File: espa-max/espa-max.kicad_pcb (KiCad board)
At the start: 2 copper layers, 44.1 x 47.5 mm, 39 parts, among them J1 Conn_01x11_Pin, J3 RJ45_LED_Shielded_x2, J5 AudioPlug2, U1 ESP32-S3-MINI-1-N8, U2 ESD7104MUTAG, U3 AP63203WU

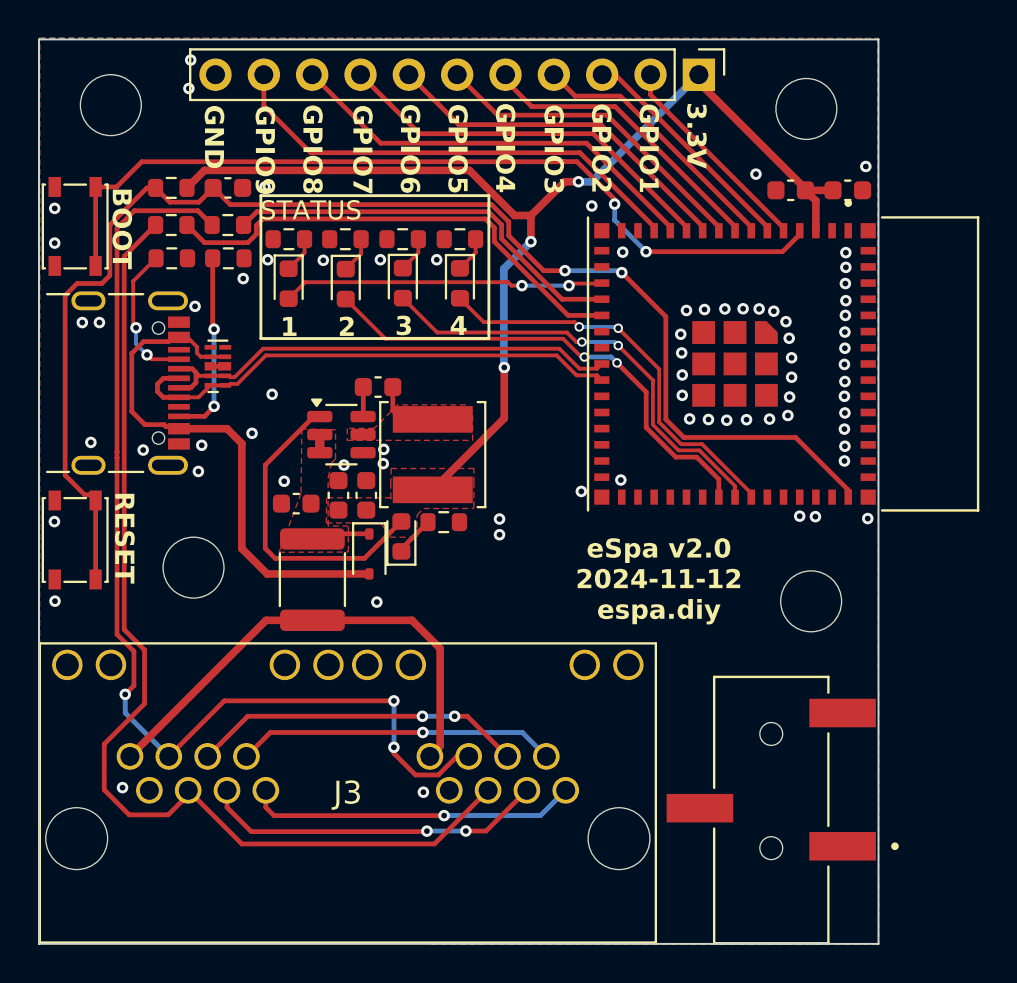
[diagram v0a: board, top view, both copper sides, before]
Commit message: Misc updates from a while back. Committing before I do an update to use smaller components.
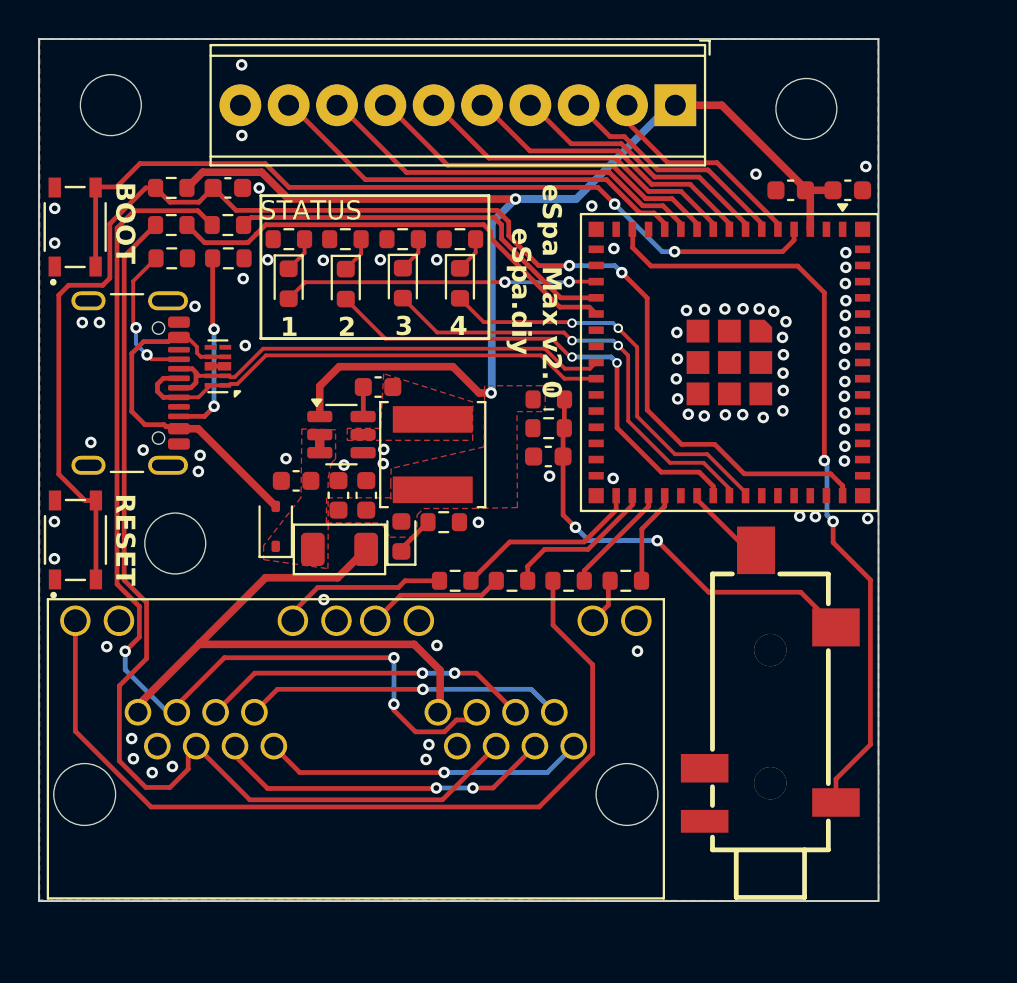
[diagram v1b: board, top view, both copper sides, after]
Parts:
- removed BOOT1: BOOT, Button_Switch_SMD:SW_SPST_PTS810
- removed F1: 30V 500mA, Fuse:Fuse_1812_4532Metric
- removed G***: LOGO, espa-logo:espa-logo-40mm
- removed H2: MountingHole, MountingHole:MountingHole_3.2mm_M3
- removed J5: AudioPlug2, PJ-320B:BOOMELE_PJ-320B
- removed RESET1: RESET, Button_Switch_SMD:SW_SPST_PTS810
- added C4: 10μF, Capacitor_SMD:C_0603_1608Metric, F.Cu at (140.2, 97.2)
- added F2: 33V 500mA, PCM_Fuse_AKL:Fuse_1206_3216Metric, F.Cu at (129.2, 102.1)
- added R11: 10kΩ, Resistor_SMD:R_0603_1608Metric, F.Cu at (140.2, 94.2)
- added R12: 10kΩ, Resistor_SMD:R_0603_1608Metric, F.Cu at (140.2, 95.8)
- added R13: 330Ω, Resistor_SMD:R_0603_1608Metric, F.Cu at (135.3, 103.8)
- added R14: 330Ω, Resistor_SMD:R_0603_1608Metric, F.Cu at (141.2, 103.8)
- added R15: 330Ω, Resistor_SMD:R_0603_1608Metric, F.Cu at (144.2, 103.8)
- added R16: 330Ω, Resistor_SMD:R_0603_1608Metric, F.Cu at (138.3, 103.8)
- added S1: BOOT, ALPS SKRPACE010:SW_SKRPACE010, F.Cu at (115.3, 85.2)
- added S2: RESET, ALPS SKRPACE010:SW_SKRPACE010, F.Cu at (115.3, 101.6)
- added U5: ESP32-S3-MINI-1U, RF_Module:ESP32-S2-MINI-1U, F.Cu at (149.7, 92.3)
- J1: value Conn_01x11_Pin -> Screw_Terminal_01x10; footprint Connector_PinHeader_2.54mm:PinHeader_1x11_P2.54mm_Vertical -> TerminalBlock_Phoenix:TerminalBlock_Phoenix_MPT-0,5-10-2.54_1x10_P2.54mm_Horizontal
- U1: value ESP32-S3-MINI-1-N8 -> KH-PJ-328-SMT; footprint ESP32-S3-MINI-1-N8:XCVR_ESP32-S3-MINI-1-N8 -> 3.5mm-connector:AUDIO-SMD_KH-PJ-328-SMT
- moved U1 17.0 mm to (151.8, 109.3), turned to 90 degrees
- moved D3 5.13 mm to (125.8, 100.9), turned to 90 degrees
- moved J3 2.36 mm to (130.1, 112.6)
- moved J1 2.03 mm to (146.8, 78.8), turned to 180 degrees
- moved H4 1.59 mm to (120.6, 101.8)
- moved C5 1.20 mm to (126.9, 98.5)
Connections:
- net RJ45-8 renamed /+12V
- J1 pad 10: /GPIO9 -> GND
- J3 pad 10: unconnected-(J3-Pad10) -> Net-(J3-Pad10)
- J3 pad 11: unconnected-(J3-Pad11) -> GND
- J3 pad 12: unconnected-(J3-Pad12) -> Net-(J3-Pad12)
- J3 pad 21: unconnected-(J3-Pad21) -> GND
- J3 pad 22: unconnected-(J3-Pad22) -> Net-(J3-Pad22)
- J3 pad 23: unconnected-(J3-Pad23) -> GND
- J3 pad 24: unconnected-(J3-Pad24) -> Net-(J3-Pad24)
- J3 pad 9: unconnected-(J3-Pad9) -> GND
- U1 pad 3: +3.3V -> GPIO10
- U1 pad 4: /GPIO0 -> unconnected-(U1-Pad4)
- U1 pad 5: /GPIO1 -> GPIO40
- U1 pad 6: /GPIO2 -> Net-(C4-Pad1)
- U1 pad 7: /GPIO3 -> unconnected-(U1-Pad7)
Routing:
- net Net-(J3-Pad24): track 0.00 -> 45.7 mm
- net GPIO10: track 0.00 -> 40.5 mm, vias 0 -> 2
- net /GPIO9: track 24.8 -> 0.00 mm
- net Net-(C4-Pad1): track 0.00 -> 22.9 mm, vias 0 -> 2
- net +3.3V: track 75.8 -> 63.2 mm, vias 3 -> 2
- net GPIO35: track 0.00 -> 9.93 mm
- net /+5V: track 27.2 -> 17.6 mm
- net Net-(J3-Pad22): track 0.00 -> 8.83 mm
- net GPIO36: track 0.00 -> 8.08 mm
- net Net-(J3-Pad12): track 0.00 -> 7.23 mm
- net GPIO37: track 0.00 -> 5.87 mm
- net GPIO38: track 0.00 -> 4.98 mm
- net /+12V: track 25.8 -> 30.7 mm
- net GPIO40: track 0.00 -> 4.56 mm
- net RJ45-6: track 55.6 -> 52.7 mm
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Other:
- board size 44.1 x 47.5 mm -> 44.1 x 45.3 mm
- board text added: "BOOT"
- board text added: "CT CLAMP"
- board text added: "LOOP"
- board text added: "RESET"
- board text added: "SPA"
- board text added: "eSpa Max v2.0 eSpa.diy"
- board text removed: "GPIO9"
- board text removed: "eSpa v2.0 2024-11-12 espa.diy"
